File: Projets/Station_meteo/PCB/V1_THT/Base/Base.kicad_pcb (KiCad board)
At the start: 2 copper layers, 87.2 x 97.9 mm, 21 parts, among them J1 Conn_02x05_Odd_Even, J10 Conn_01x04_Pin, J2 Conn_02x04_Odd_Even, J3 Conn_02x06_Odd_Even, J4 Conn_02x06_Odd_Even, J5 Screw_Terminal_01x03_2.54mm [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, J6 Screw_Terminal_01x03_2.54mm [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, J7 Screw_Terminal_01x04, J8 Screw_Terminal_01x03_2.54mm [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, J9 Screw_Terminal_01x04, U1 ATmega328P-P, U2 NRF24L01_Breakout, Y1 Crystal

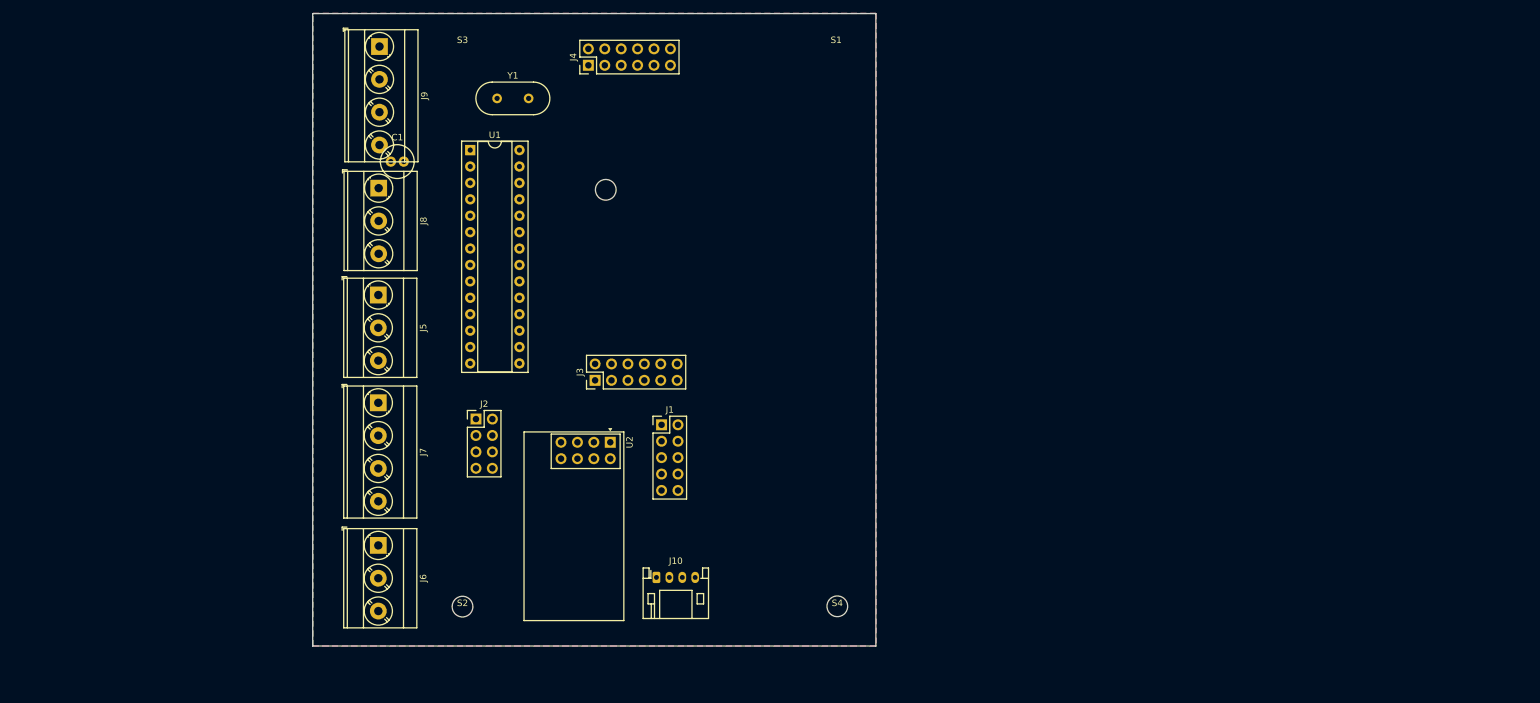
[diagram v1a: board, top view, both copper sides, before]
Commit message: Update PCB Base
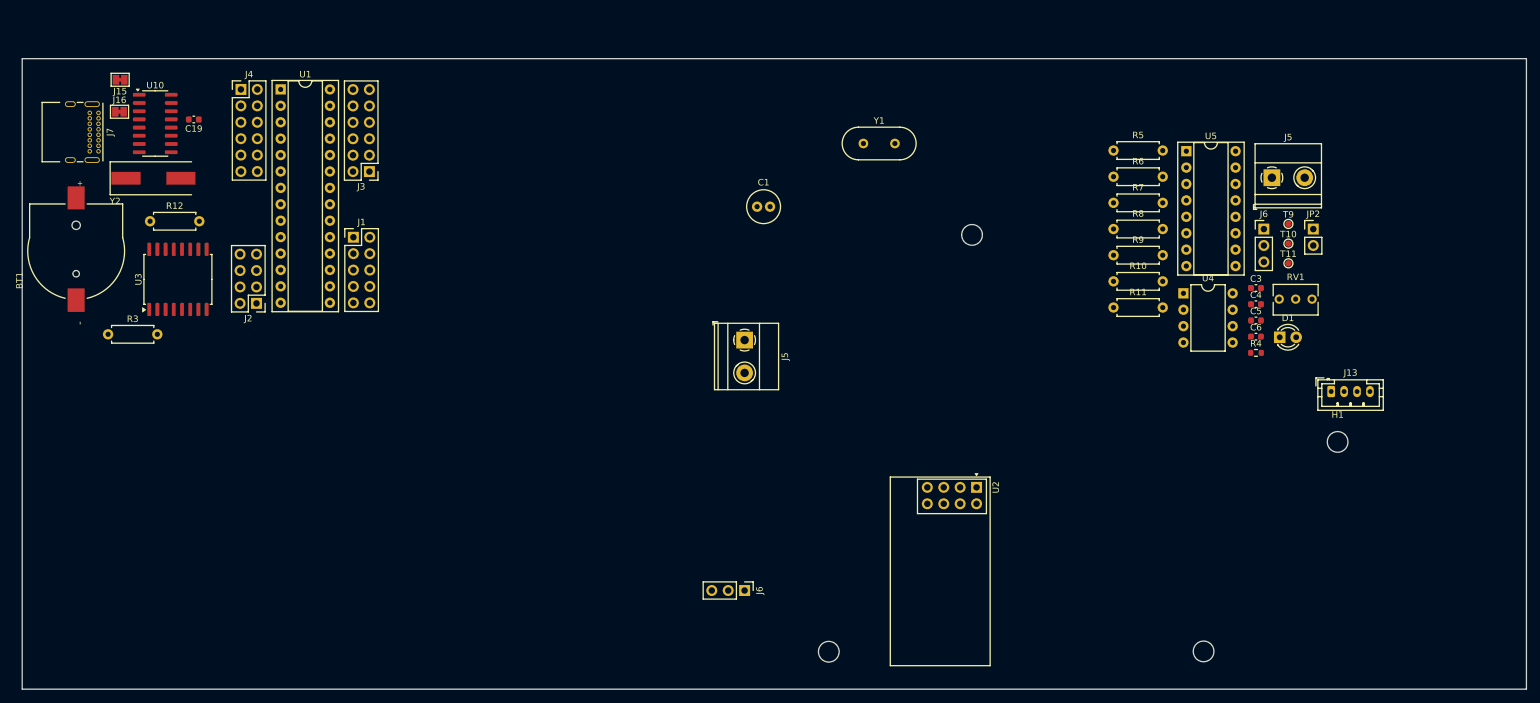
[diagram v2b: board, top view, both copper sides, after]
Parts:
- removed J10: Conn_01x04_Pin, Connector_JST:JST_PH_S4B-PH-K_1x04_P2.00mm_Horizontal
- removed J8: Screw_Terminal_01x03_2.54mm [CREPP], TerminalBlock_Phoenix:TerminalBlock_Phoenix_MKDS-3-3-5.08_1x03_P5.08mm_Horizontal
- removed J9: Screw_Terminal_01x04, TerminalBlock_Phoenix:TerminalBlock_Phoenix_MKDS-3-4-5.08_1x04_P5.08mm_Horizontal
- removed S2, S3, S4: ~, Spacers:Spacer_M3_20mm
- added BT1: Battery_Cell, CREPP_Batteries_holders:MPD_BC501SM-TR, F.Cu at (71.9, 64.0)
- added C19: 100nF, Capacitor_SMD:C_0603_1608Metric, F.Cu at (90.1, 43.6)
- added C3: 100nF, Capacitor_SMD:C_0603_1608Metric, F.Cu at (254.5, 69.7)
- added C4: 100nF, Capacitor_SMD:C_0603_1608Metric, F.Cu at (254.5, 72.2)
- added C5: 100nF, Capacitor_SMD:C_0603_1608Metric, F.Cu at (254.5, 74.8)
- added C6: 100nF, Capacitor_SMD:C_0603_1608Metric, F.Cu at (254.5, 77.3)
- added D1: LED, LED_THT:LED_D3.0mm, F.Cu at (258.2, 77.4)
- added H1: MountingHole_Pad, MountingHole:MountingHole_3.2mm_M3, F.Cu at (267.1, 93.6)
- added J13: JST_Connector, Connector_JST:JST_PH_B4B-PH-K_1x04_P2.00mm_Vertical, F.Cu at (266.1, 85.8)
- added J15: SolderJumper_2_Bridged, Jumper:SolderJumper-2_P1.3mm_Bridged_Pad1.0x1.5mm, F.Cu at (78.7, 37.5)
- added J16: SolderJumper_2_Bridged, Jumper:SolderJumper-2_P1.3mm_Bridged_Pad1.0x1.5mm, F.Cu at (78.6, 42.5)
- added J5: Screw_Terminal_01x02_2.54mm, TerminalBlock_Phoenix:TerminalBlock_Phoenix_MKDS-1,5-2-5.08_1x02_P5.08mm_Horizontal, F.Cu at (256.9, 52.7)
- added J6: Conn_01x03_Pin, Connector_PinHeader_2.54mm:PinHeader_1x03_P2.54mm_Vertical, F.Cu at (255.7, 60.6)
- added JP2: Jumper, Connector_PinHeader_2.54mm:PinHeader_1x02_P2.54mm_Vertical, F.Cu at (263.4, 60.6)
- added JP3: Jumper_2.54mm_blue, CREPP_Jumpers:Jumper_2.54mm_blue, F.Cu at (232.7, 76.6)
- added R10: 10k, Resistor_THT:R_Axial_DIN0207_L6.3mm_D2.5mm_P7.62mm_Horizontal, F.Cu at (232.4, 68.7)
- added R11: 100k, Resistor_THT:R_Axial_DIN0207_L6.3mm_D2.5mm_P7.62mm_Horizontal, F.Cu at (232.4, 72.8)
- added R12: 4.7k, Resistor_THT:R_Axial_DIN0207_L6.3mm_D2.5mm_P7.62mm_Horizontal, F.Cu at (83.3, 59.4)
- added R3: 4.7k, Resistor_THT:R_Axial_DIN0207_L6.3mm_D2.5mm_P7.62mm_Horizontal, F.Cu at (76.8, 76.9)
- added R4: R_10K_SMD_0603, Resistor_SMD:R_0603_1608Metric, F.Cu at (254.5, 79.8)
- added R5: 100k, Resistor_THT:R_Axial_DIN0207_L6.3mm_D2.5mm_P7.62mm_Horizontal, F.Cu at (232.4, 48.5)
- added R6: 10k, Resistor_THT:R_Axial_DIN0207_L6.3mm_D2.5mm_P7.62mm_Horizontal, F.Cu at (232.4, 52.5)
- added R7: 10k, Resistor_THT:R_Axial_DIN0207_L6.3mm_D2.5mm_P7.62mm_Horizontal, F.Cu at (232.4, 56.6)
- added R8: 10k, Resistor_THT:R_Axial_DIN0207_L6.3mm_D2.5mm_P7.62mm_Horizontal, F.Cu at (232.4, 60.6)
- added R9: 270, Resistor_THT:R_Axial_DIN0207_L6.3mm_D2.5mm_P7.62mm_Horizontal, F.Cu at (232.4, 64.7)
- added RV1: R_Potentiometer, Potentiometer_THT:Potentiometer_Bourns_3266Y_Vertical, F.Cu at (263.2, 71.5)
- added S1: ~, CREPP_Spacers:Spacer_M3_MF_05mm, F.Cu at (259.6, 86.6)
- added S5: ~, CREPP_Spacers:Spacer_M3_MF_05mm, F.Cu at (259.6, 93.8)
- added S6: ~, CREPP_Spacers:Spacer_M3_MF_05mm, F.Cu at (259.6, 101.0)
- added S7: ~, CREPP_Spacers:Spacer_M3_MF_05mm, F.Cu at (259.6, 108.2)
- added T10: TP, TestPoint:TestPoint_Pad_D1.0mm, F.Cu at (259.5, 62.9)
- added T11: TP, TestPoint:TestPoint_Pad_D1.0mm, F.Cu at (259.5, 65.9)
- added T9: TP, TestPoint:TestPoint_Pad_D1.0mm, F.Cu at (259.5, 59.8)
- added U10: CH340G, Package_SO:SOIC-16_3.9x9.9mm_P1.27mm, F.Cu at (84.1, 44.3)
- added U3: DS3231M, Package_SO:SOIC-16W_7.5x10.3mm_P1.27mm, F.Cu at (87.6, 68.4)
- added U4: LM358, Package_DIP:DIP-8_W7.62mm, F.Cu at (243.3, 70.6)
- added U5: 74HC123, Package_DIP:DIP-16_W7.62mm_Socket, F.Cu at (243.7, 48.6)
- added Y2: 12MHz, Crystal:Crystal_SMD_HC49-SD, F.Cu at (83.8, 52.8)
- J5: value Screw_Terminal_01x03_2.54mm [CREPP] -> Screw_Terminal_01x02_2.54mm; footprint TerminalBlock_Phoenix:TerminalBlock_Phoenix_MKDS-3-3-5.08_1x03_P5.08mm_Horizontal -> TerminalBlock_Phoenix:TerminalBlock_Phoenix_MKDS-1,5-2-5.08_1x02_P5.08mm_Horizontal
- J6: value Screw_Terminal_01x03_2.54mm [CREPP] -> Conn_01x03_Pin; footprint TerminalBlock_Phoenix:TerminalBlock_Phoenix_MKDS-3-3-5.08_1x03_P5.08mm_Horizontal -> Connector_PinHeader_2.54mm:PinHeader_1x03_P2.54mm_Vertical
- J7: value Screw_Terminal_01x04 -> USB_C_Receptacle; footprint TerminalBlock_Phoenix:TerminalBlock_Phoenix_MKDS-3-4-5.08_1x04_P5.08mm_Horizontal -> CREPP_Connectors_USB:USB_C_Receptacle_GCT_USB4085
- S1: footprint Spacers:Spacer_M3_20mm -> CREPP_Spacers:Spacer_M3_MF_05mm
- moved J7 62.4 mm to (75.3, 42.6)
- moved H4 57.1 mm to (246.4, 126.0)
- moved U2 57.1 mm to (211.2, 100.6)
- moved C1 57.1 mm to (177.3, 57.1)
- moved H3 57.1 mm to (188.4, 126.0)
- moved J6 57.1 mm to (175.3, 116.6)
- moved S1 57.1 mm to (246.2, 38.8)
- moved Y1 57.1 mm to (193.7, 47.4)
- moved J5 57.1 mm to (175.3, 77.8)
- moved H2 57.1 mm to (210.5, 61.5)
- moved J1 55.8 mm to (114.8, 61.9)
- moved J4 53.9 mm to (97.4, 39.0), turned to 0 degrees
- moved J3 47.6 mm to (117.3, 51.7), turned to 180 degrees
- moved J2 38.4 mm to (99.8, 72.1), turned to 180 degrees
- moved U1 30.8 mm to (103.5, 39.0)
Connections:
- J5 pad 1: unconnected-(J5-Pin_1-Pad1) -> Net-(J5-Pin_1)
- J5 pad 2: unconnected-(J5-Pin_2-Pad2) -> Net-(J5-Pin_2)
- J6 pad 1: unconnected-(J6-Pin_1-Pad1) -> Net-(J5-Pin_2)
- J6 pad 2: unconnected-(J6-Pin_2-Pad2) -> /Anemometer1/Anemo_{signal}
- J6 pad 3: unconnected-(J6-Pin_3-Pad3) -> Net-(J5-Pin_1)
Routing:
- removed copper zone on B.Cu, net GND
- removed copper zone on F.Cu, net GND
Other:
- board size 87.2 x 97.9 mm -> 232.8 x 97.6 mm
